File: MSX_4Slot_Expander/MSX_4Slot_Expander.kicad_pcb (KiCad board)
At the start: 2 copper layers, 119 x 174 mm, 67 parts, among them CN1 MSX_SLOT_CON-msxmakers, CN2 Conn_02x25_Odd_Even_MountingP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, CN3 Conn_02x25_Odd_Even_MountingP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, CN4 Conn_02x25_Odd_Even_MountingP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, CN5 Conn_02x25_Odd_Even_MountingP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, SW1 SW_Push_DPDT, SW2 SW_Push_DPDT, SW3 SW_Push_DPDT, SW4 SW_Push_DPDT, U1 74LS30, U10 74HC245, U11 74HCT541, U12 74HCT541, U13 74HCT541, U2 74LS30, U3 74LS32, U4 74LS240, U5 74LS273, U6 74LS153, U7 74LS139, U8 74HCT32, U9 74LS08

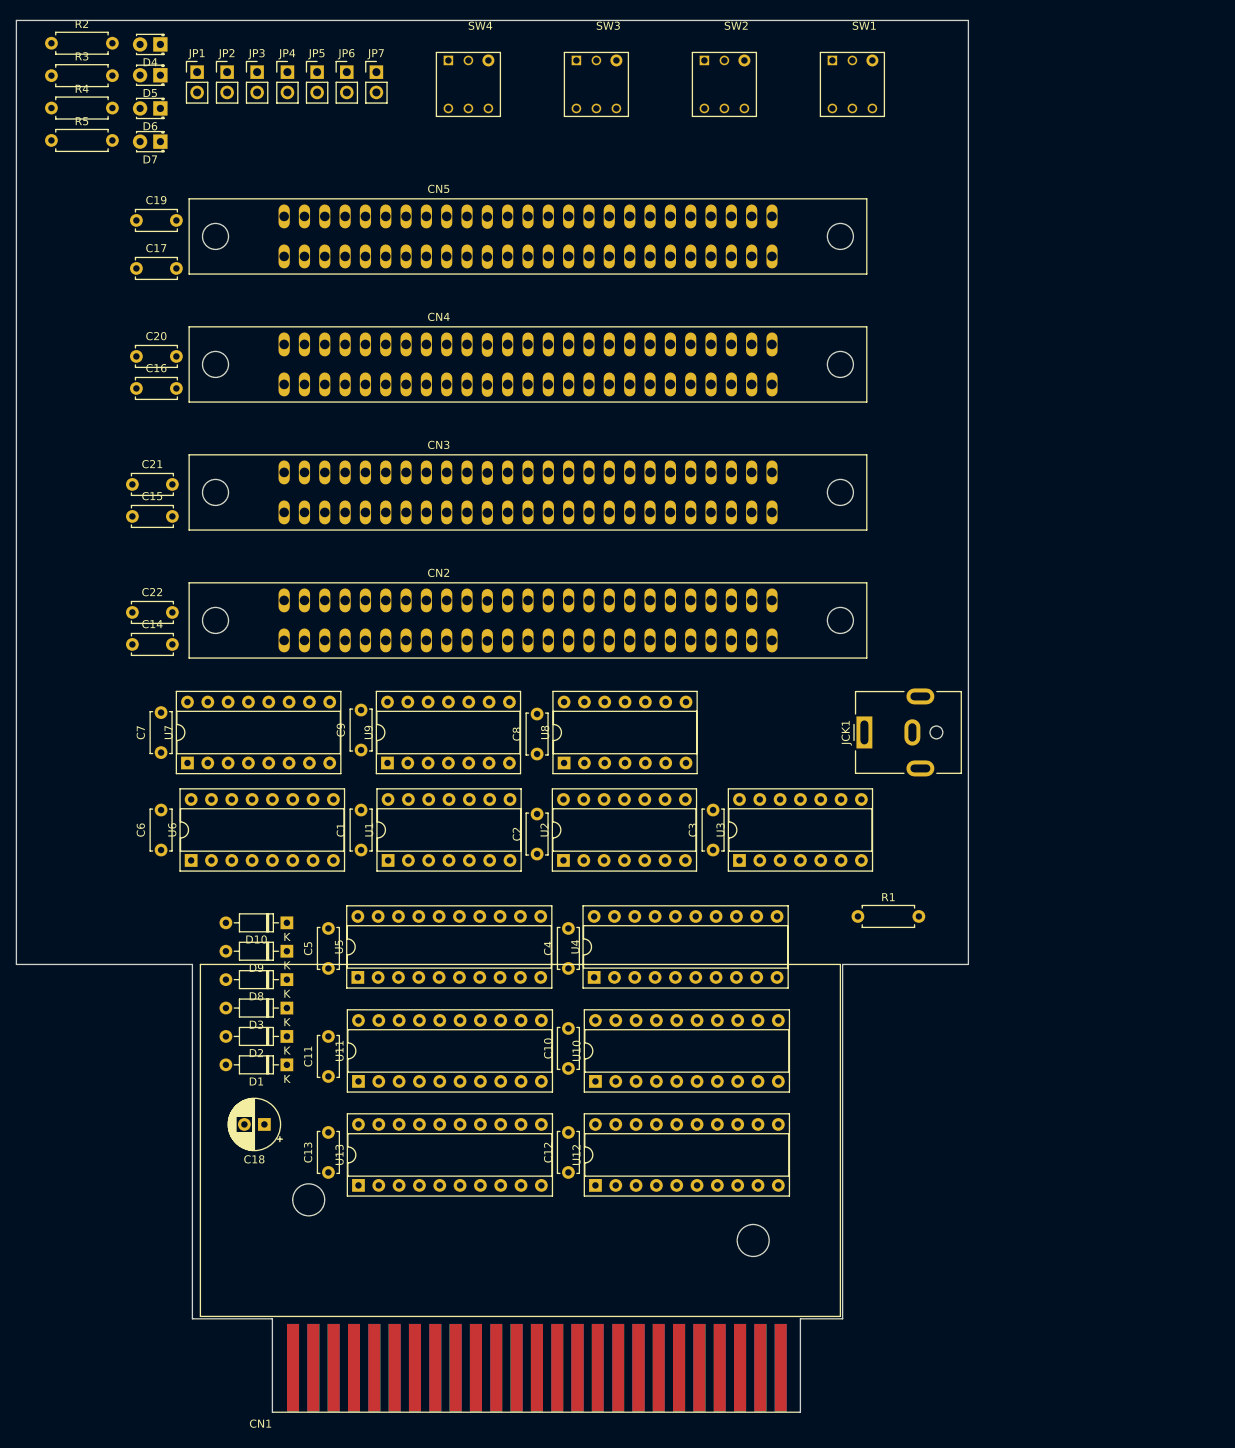
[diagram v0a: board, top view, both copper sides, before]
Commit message: Add files via upload
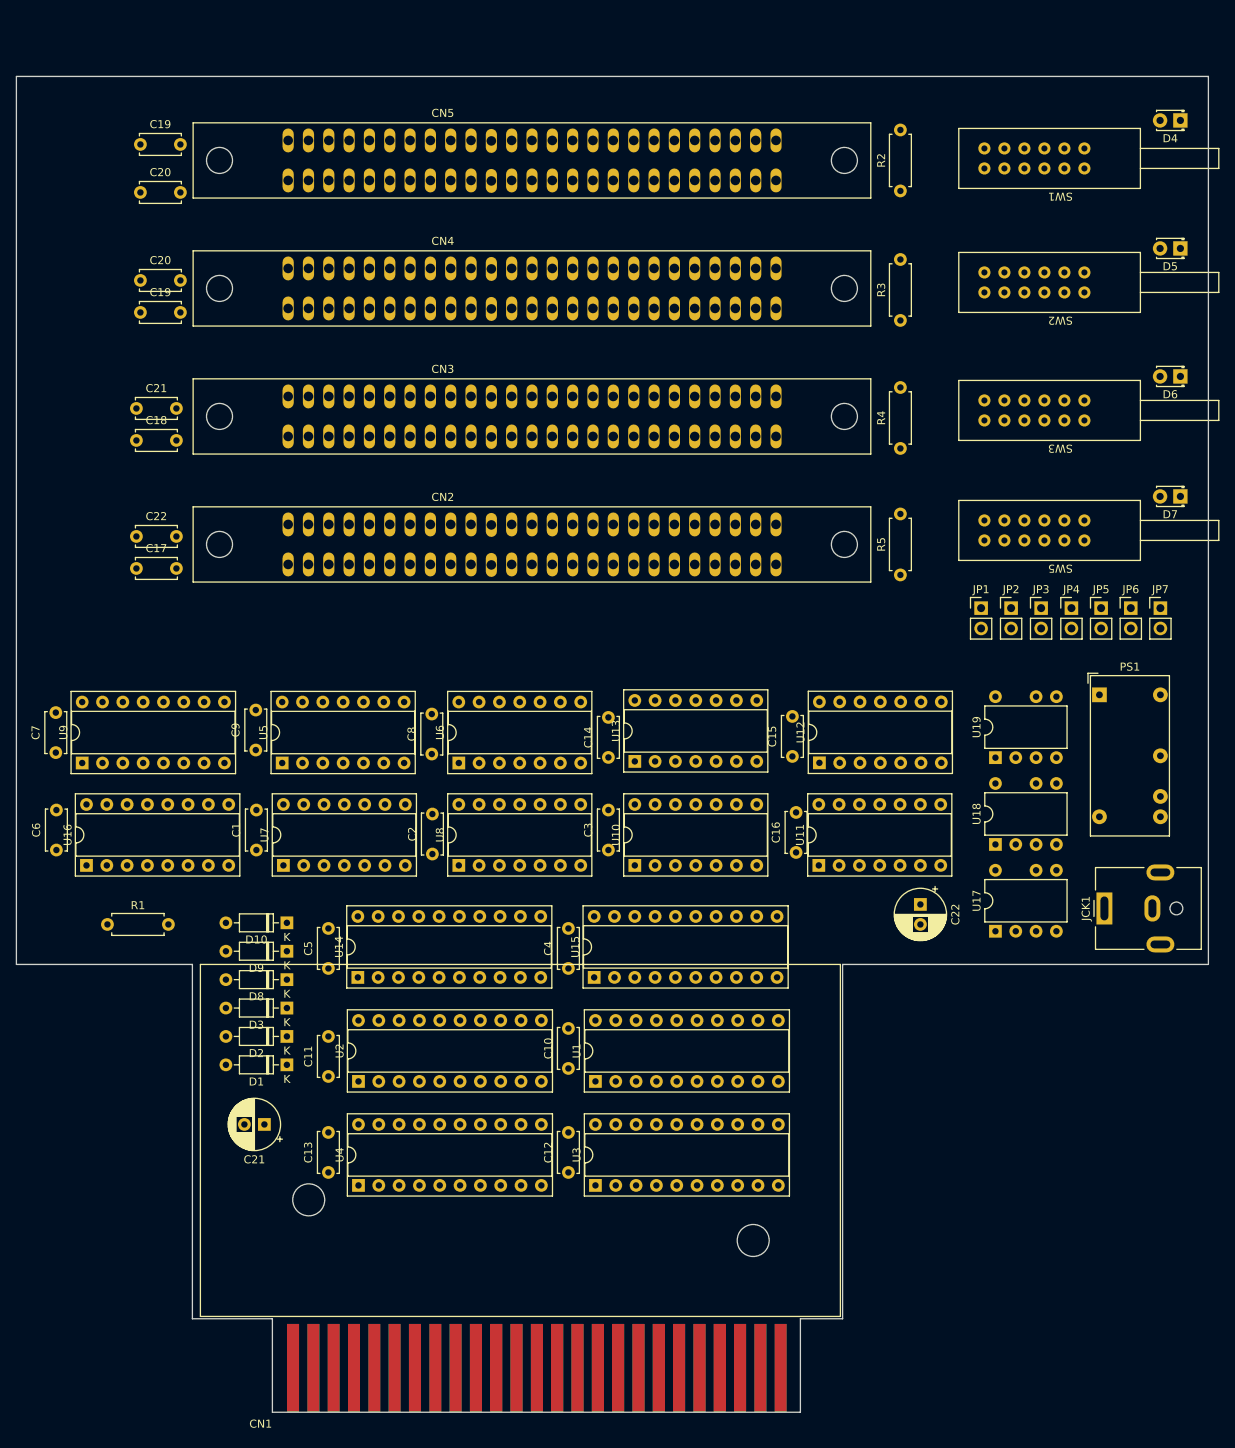
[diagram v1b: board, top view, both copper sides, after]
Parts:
- removed SW4: SW_Push_DPDT, MSX:SW_PUSH_E-Switch_TL2285_DPDT
- added C14: 104, Capacitor_THT:C_Disc_D5.0mm_W2.5mm_P5.00mm, F.Cu at (108.0, 142.1)
- added C15: 104, Capacitor_THT:C_Disc_D5.0mm_W2.5mm_P5.00mm, F.Cu at (131.0, 142.0)
- added C16: 104, Capacitor_THT:C_Disc_D5.0mm_W2.5mm_P5.00mm, F.Cu at (131.5, 154.0)
- added C22: 100uF, Capacitor_THT:CP_Radial_D6.3mm_P2.50mm, F.Cu at (147.0, 160.5)
- added PS1: IH0512D, Converter_DCDC:Converter_DCDC_XP_POWER-IHxxxxD_THT, F.Cu at (169.4, 134.3)
- added SW5: SW_Push_4PDT, MSX:Push Switch 4P2T SPUJ193700, F.Cu at (167.5, 112.5)
- added U11: 74LS11, Package_DIP:DIP-14_W7.62mm_Socket, F.Cu at (134.3, 155.6)
- added U12: 74LS08, Package_DIP:DIP-14_W7.62mm_Socket, F.Cu at (134.4, 142.8)
- added U13: 74LS32, Package_DIP:DIP-14_W7.62mm_Socket, F.Cu at (111.3, 142.6)
- added U17: AQH0223, Package_DIP:DIP-8-N7_W7.62mm, F.Cu at (156.4, 163.8)
- added U18: AQH0223, Package_DIP:DIP-8-N7_W7.62mm, F.Cu at (156.4, 153.0)
- added U19: AQH0223, Package_DIP:DIP-8-N7_W7.62mm, F.Cu at (156.4, 142.2)
- SW1, SW2, SW3: value SW_Push_DPDT -> SW_Push_4PDT; footprint MSX:SW_PUSH_E-Switch_TL2285_DPDT -> MSX:Push Switch 4P2T SPUJ193700
- moved D7 135.0 mm to (179.5, 109.5)
- moved D6 131.8 mm to (179.5, 94.5)
- moved D5 129.3 mm to (179.5, 78.5)
- moved D4 127.9 mm to (179.5, 62.5)
- moved R5 119.2 mm to (144.5, 119.3), turned to 90 degrees
- moved JP6 118.7 mm to (173.3, 123.5)
- moved JP1 118.7 mm to (154.6, 123.5)
- moved JP2 118.7 mm to (158.3, 123.5)
- moved JP3 118.7 mm to (162.1, 123.5)
- moved JP4 118.7 mm to (165.9, 123.5)
- moved JP5 118.7 mm to (169.6, 123.5)
- moved JP7 118.7 mm to (177.0, 123.5)
- moved R4 114.3 mm to (144.5, 103.5), turned to 90 degrees
- moved R3 110.4 mm to (144.5, 87.5), turned to 90 degrees
- moved R2 107.7 mm to (144.5, 71.3), turned to 90 degrees
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- renumbered C14 to C17, C15 to C18, C16 to C19, C17 to C20, C18 to C21, U10 to U1, U3 to U10, U5 to U14, U4 to U15, U6 to U16, U11 to U2, U12 to U3, U13 to U4, U9 to U5, U8 to U6, U1 to U7, U2 to U8, U7 to U9
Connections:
- C10 pad 1: +5V -> +5VS
- C11 pad 1: +5V -> +5VS
- C12 pad 1: +5V -> +5VS
- C13 pad 1: +5V -> +5VS
- C21 pad 1: +5V -> +5VS
- C7 pad 1: +5V -> +5VS
- C8 pad 1: +5V -> +5VS
- C9 pad 1: +5V -> +5VS
- CN2 pad 10: BXDIR -> BXDIR0
- CN2 pad 48: +12V -> +12VS0
- CN2 pad 50: -12V -> -12VS0
- CN3 pad 10: BXDIR -> BXDIR1
- CN3 pad 48: +12V -> +12VS1
- CN3 pad 50: -12V -> -12VS1
- CN4 pad 10: BXDIR -> BXDIR2
- CN4 pad 48: +12V -> +12VS2
- CN4 pad 50: -12V -> -12VS2
- CN5 pad 10: BXDIR -> BXDIR3
- CN5 pad 48: +12V -> +12VS3
- CN5 pad 50: -12V -> -12VS3
- JCK1 pad 1: +5VS -> Net-(PS1-+Vin)
- R2 pad 1: +5V -> +5VS
- R3 pad 1: +5V -> +5VS
- R4 pad 1: +5V -> +5VS
- R5 pad 1: +5V -> +5VS
- SW1 pad 1: unconnected-(SW1-A-Pad1) -> SLTX1
- SW1 pad 2: Net-(JP1-A) -> Net-(JP2-A)
- SW1 pad 3: SLTX0 -> unconnected-(SW1-C-Pad3)
- SW1 pad 6: +5VS0 -> +5VS1
- SW2 pad 1: unconnected-(SW2-A-Pad1) -> SLTX2
- SW2 pad 2: Net-(JP2-A) -> Net-(JP3-A)
- SW2 pad 3: SLTX1 -> unconnected-(SW2-C-Pad3)
- SW2 pad 6: +5VS1 -> +5VS2
- SW3 pad 1: unconnected-(SW3-A-Pad1) -> SLTX3
- SW3 pad 2: Net-(JP3-A) -> Net-(JP4-A)
- SW3 pad 3: SLTX2 -> unconnected-(SW3-C-Pad3)
- SW3 pad 6: +5VS2 -> +5VS3
- U10 pad 14: +5V -> +5VS
- U10 pad 9: Net-(D1-A) -> Net-(U10-Pad9)
- U14 pad 20: +5V -> +5VS
- U15 pad 20: +5V -> +5VS
- U16 pad 16: +5V -> +5VS
- U7 pad 14: +5V -> +5VS
- U8 pad 14: +5V -> +5VS
- U9 pad 16: +5V -> +5VS
- U9 pad 5: Net-(D1-K) -> Net-(U9A-O1)
- U9 pad 6: Net-(D2-K) -> Net-(U9A-O2)
- U9 pad 7: Net-(D3-K) -> Net-(U9A-O3)
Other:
- board size 119 x 174 mm -> 149 x 167 mm
